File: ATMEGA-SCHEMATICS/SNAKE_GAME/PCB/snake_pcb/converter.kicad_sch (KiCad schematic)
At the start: 8 parts, among them J3 USB_A, U5 FT232RL

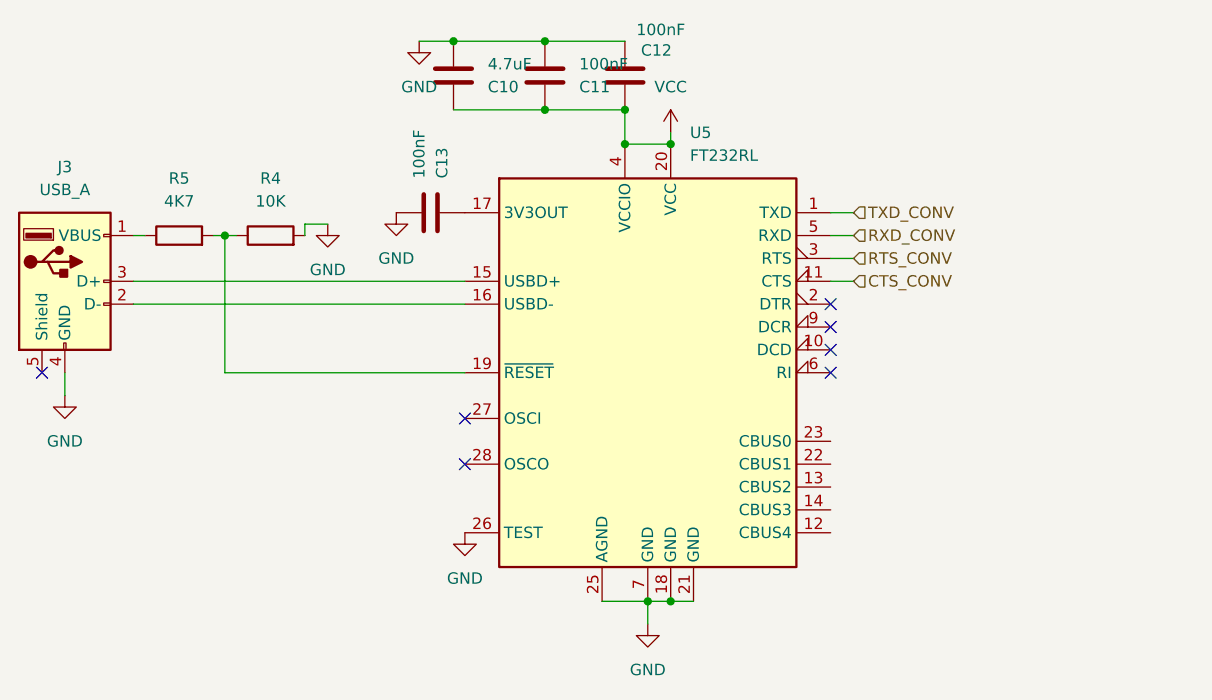
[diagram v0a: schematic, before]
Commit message: .
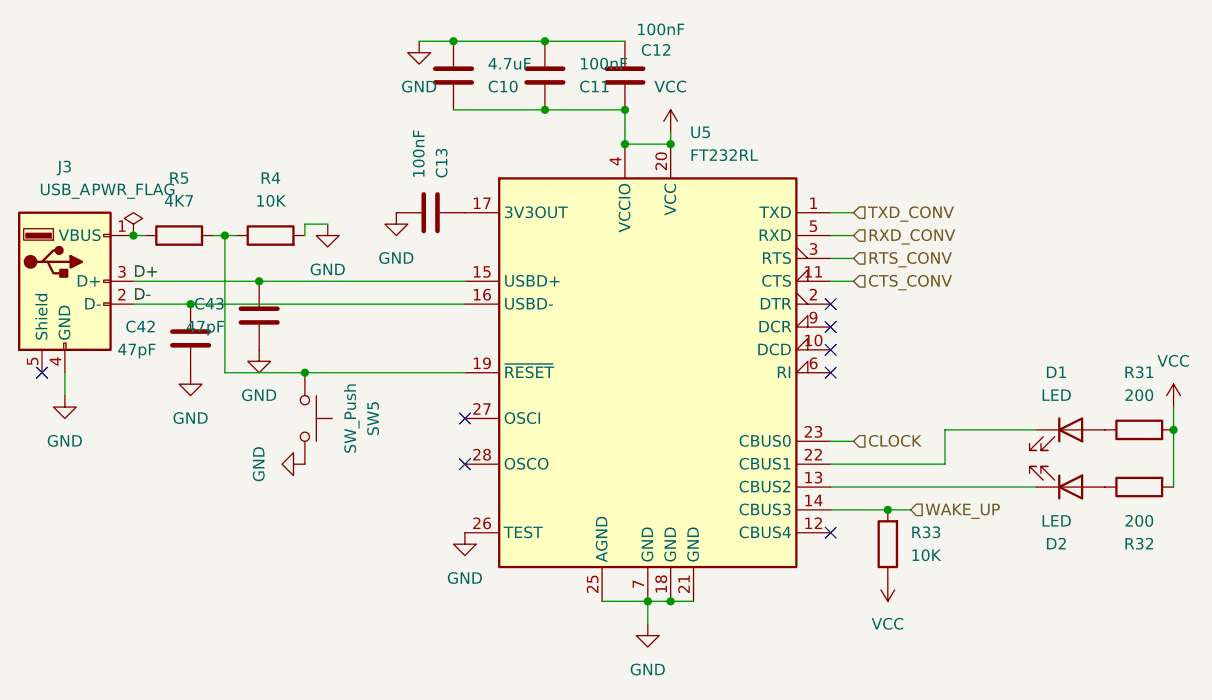
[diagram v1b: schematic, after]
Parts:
- added C42, C43: 47pF, Capacitor_THT:C_Disc_D7.5mm_W5.0mm_P5.00mm, symbol Device:C
- added D1, D2: LED, LED_THT:LED_D1.8mm_W3.3mm_H2.4mm, symbol Device:LED
- added R31, R32: 200, Resistor_THT:R_Axial_DIN0207_L6.3mm_D2.5mm_P10.16mm_Horizontal, symbol Device:R
- added R33: 10K, Resistor_THT:R_Axial_DIN0207_L6.3mm_D2.5mm_P10.16mm_Horizontal, symbol Device:R
- added SW5: SW_Push, Button_Switch_THT:SW_PUSH_1P1T_6x3.5mm_H4.3_APEM_MJTP1243, symbol Switch:SW_Push
- C10, C11, C12, C13: footprint (none) -> Capacitor_THT:C_Disc_D7.5mm_W5.0mm_P5.00mm
- J3: footprint (none) -> Connector_USB:USB_B_Lumberg_2411_02_Horizontal
- R4, R5: footprint (none) -> Resistor_THT:R_Axial_DIN0207_L6.3mm_D2.5mm_P10.16mm_Horizontal
- U5: footprint Package_SO:SSOP-28_5.3x10.2mm_P0.65mm -> Package_DIP:DIP-28_W15.24mm_LongPads
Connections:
- net GND: now also C42.2, C43.2, SW5.2
- net VCC: now also R31.2, R32.2, R33.1
- net at U5.13 (CBUS2): now also D2.1 (K)
- net WAKE_UP: now reaches U5.14 (CBUS3)
- net WAKE_UP: now also R33.2
- net D+: now reaches J3.3 (D+), U5.15 (USBD+)
- net D+: now also C43.1
- net D-: now reaches J3.2 (D-), U5.16 (USBD-)
- net D-: now also C42.1
- net at R4.1, R5.2, U5.19 (~{RESET}): now also SW5.1
- net at U5.22 (CBUS1): now also D1.1 (K)
- net CLOCK: now reaches U5.23 (CBUS0)
- new net: D2.2 (A), R32.1
- new net: D1.2 (A), R31.1
- no-connect marks 7 -> 8
